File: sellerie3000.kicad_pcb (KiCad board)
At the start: 2 copper layers, 25.4 x 10.2 mm, 19 parts, among them J1 USB_C_Receptacle, J2 Conn_01x04, J3 Conn_01x02, J4 Conn_01x02, U1 FT230XQ-R

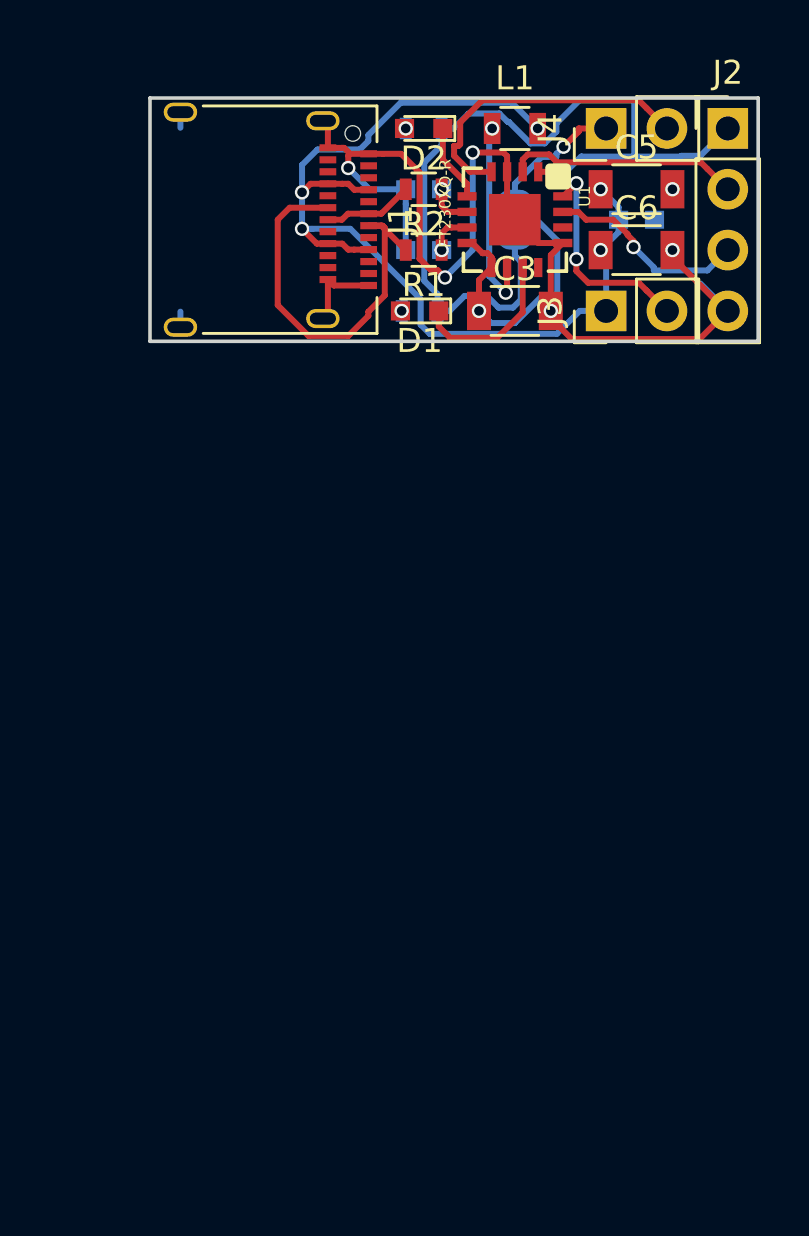
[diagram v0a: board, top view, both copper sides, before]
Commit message: wow much update many unfinished
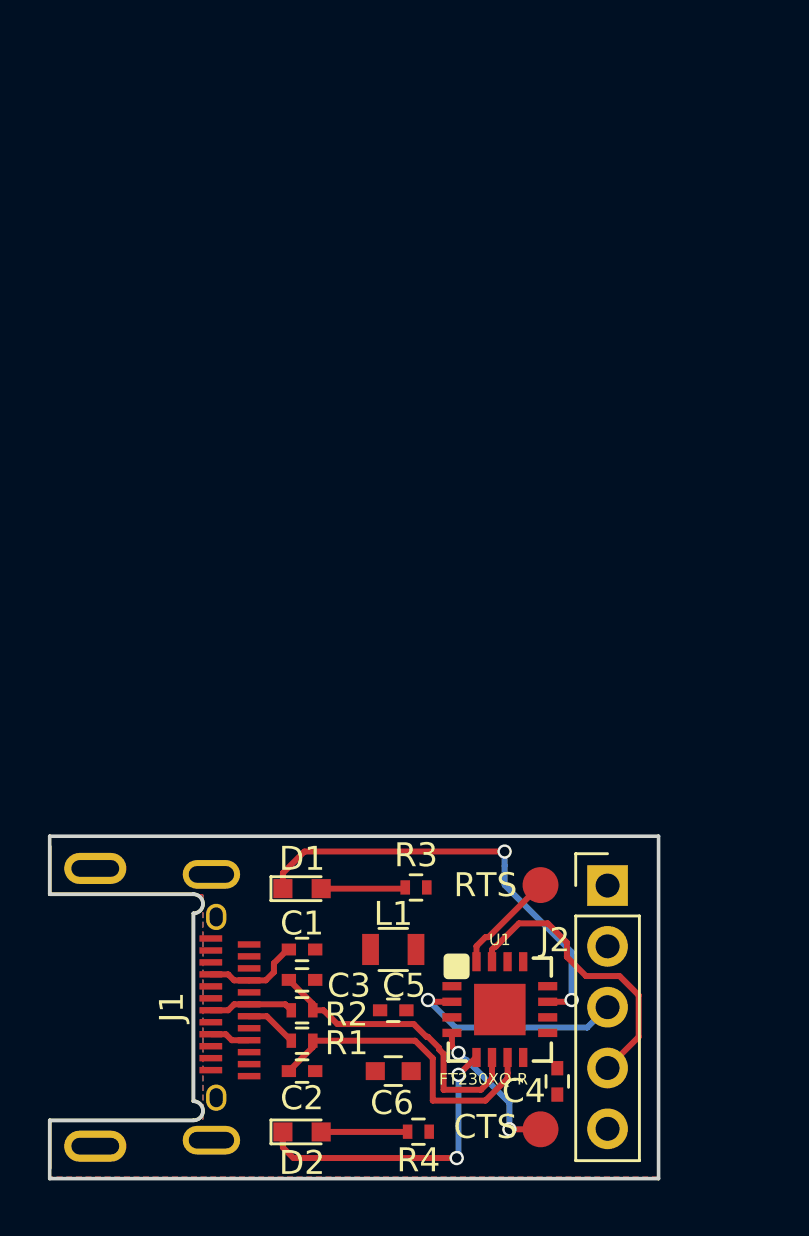
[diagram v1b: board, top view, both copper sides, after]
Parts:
- removed J3, J4: Conn_01x02, Pin_Headers:Pin_Header_Straight_1x02_Pitch2.54mm
- removed JP1: VMODE, sellerie3000:Solder_Jumper
- added CTS: CTS, Measurement_Points:Measurement_Point_Round-SMD-Pad_Small, F.Cu at (139.5, 143.4)
- added RTS: RTS, Measurement_Points:Measurement_Point_Round-SMD-Pad_Small, F.Cu at (139.5, 133.2)
- C1: value 47pF -> 10nF; footprint Capacitors_SMD:C_0603 -> Capacitors_SMD:C_0402; moved to F.Cu
- C2: footprint Capacitors_SMD:C_0603 -> Capacitors_SMD:C_0402; moved to F.Cu
- C3: value 100nF -> 47pF; footprint Capacitors_SMD:C_1206 -> Capacitors_SMD:C_0402
- C4: value 10nF -> 100nF; footprint Capacitors_SMD:C_0603 -> Capacitors_SMD:C_0402; moved to F.Cu
- C5: footprint Capacitors_SMD:C_1206 -> Capacitors_SMD:C_0402
- C6: footprint Capacitors_SMD:C_1206 -> Capacitors_SMD:C_0603
- D1: value RXLED -> RX
- D2: value TXLED -> TX
- J1: footprint Connectors_USB:USB_C_Receptacle_Amphenol_12401610E4-2A -> DX07B024JJ3:DX07B024JJ3
- J2: value Conn_01x04 -> Conn_01x05; footprint Pin_Headers:Pin_Header_Straight_1x04_Pitch2.54mm -> Pin_Headers:Pin_Header_Straight_1x05_Pitch2.54mm
- R1, R2: footprint Resistors_SMD:R_0603 -> Resistors_SMD:R_0402
- R3, R4: footprint Resistors_SMD:R_0603 -> Resistors_SMD:R_0402; moved to F.Cu
- moved D2 42.2 mm to (129.5, 143.5), turned to 0 degrees
- moved R4 41.9 mm to (134.4, 143.5)
- moved C4 36.1 mm to (140.2, 141.4), turned to 270 degrees
- moved C5 35.8 mm to (133.3, 138.4)
- moved C6 35.8 mm to (133.3, 141.0)
- moved R2 34.7 mm to (129.5, 138.4)
- moved C2 34.7 mm to (129.5, 141.0), turned to 0 degrees
- moved L1 34.7 mm to (133.3, 135.9)
- moved R1 33.4 mm to (129.5, 139.7)
- moved U1 33.0 mm to (137.8, 138.4), turned to 0 degrees
- moved J1 32.9 mm to (125.8, 138.3)
- moved C1 32.2 mm to (129.5, 135.9), turned to 0 degrees
- moved J2 32.0 mm to (142.3, 133.2)
- moved C3 29.3 mm to (129.5, 137.2)
- moved D1 24.6 mm to (129.5, 133.3), turned to 0 degrees
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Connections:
- net CBUS1 renamed /CBUS1
- net CBUS2 renamed /CBUS2
- net Net-(C2-Pad1) renamed /USBDM
- C3 pad 1: 3V3 -> /USBDP
- C4 pad 1: VCC -> 3V3
- J1 pad A4: VCC -> Net-(C1-Pad1)
- J1 pad A9: VCC -> Net-(C1-Pad1)
- J1 pad B4: VCC -> Net-(C1-Pad1)
- J1 pad B9: VCC -> Net-(C1-Pad1)
- J2 pad 1: VCCIO -> VCC
- J2 pad 2: RX -> 3V3
- J2 pad 3: TX -> RX
- J2 pad 4: GND -> TX
- L1 pad 1: Net-(L1-Pad1) -> VCC
- L1 pad 2: VCC -> Net-(C1-Pad1)
- R2 pad 1: Net-(C1-Pad1) -> /USBDP
- R3 pad 1: VCCIO -> 3V3
- R4 pad 1: VCCIO -> 3V3
- U1 pad 1: VCCIO -> 3V3
- U1 pad 10: Net-(L1-Pad1) -> VCC
- U1 pad 16: RTS -> /RTS
- U1 pad 4: CTS -> /CTS
- U1 pad 6: Net-(C1-Pad1) -> /USBDP
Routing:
- net GND: track 50.3 -> 0.00 mm, vias 6 -> 0
- net VCC: track 41.7 -> 0.00 mm, vias 5 -> 0
- net VCCIO: track 36.0 -> 0.00 mm, vias 1 -> 0
- net 3V3: track 18.2 -> 0.00 mm, vias 2 -> 0
- net Net-(J1-PadA7): track 17.2 -> 2.18 mm
- net CTS: track 13.0 -> 0.00 mm
- net /USBDP: track 0.00 -> 12.5 mm
- net /CBUS1: track 6.66 -> 18.7 mm, vias 0 -> 2
- net /USBDM: track 1.86 -> 13.1 mm, vias 1 -> 0
- net /CBUS2: track 3.25 -> 12.6 mm, vias 0 -> 2
- net RTS: track 8.93 -> 0.00 mm, vias 2 -> 0
- net Net-(L1-Pad1): track 8.27 -> 0.00 mm, vias 2 -> 0
- net /CTS: track 0.00 -> 6.35 mm, vias 0 -> 2
- net /RTS: track 0.00 -> 4.38 mm
- net Net-(C1-Pad1): track 1.86 -> 5.82 mm, vias 1 -> 0
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- added copper zone on F.Cu, net GND
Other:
- board size 25.4 x 10.2 mm -> 25.4 x 14.3 mm

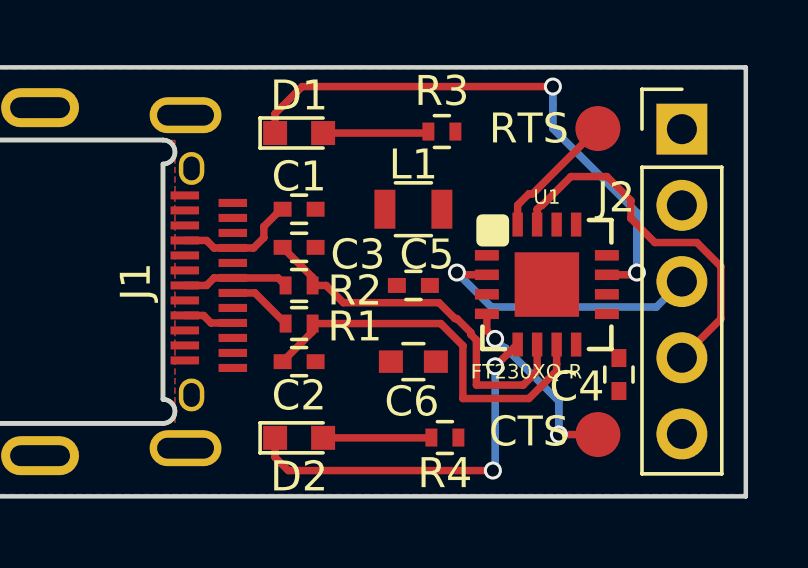
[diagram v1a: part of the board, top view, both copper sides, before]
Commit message: nearly done
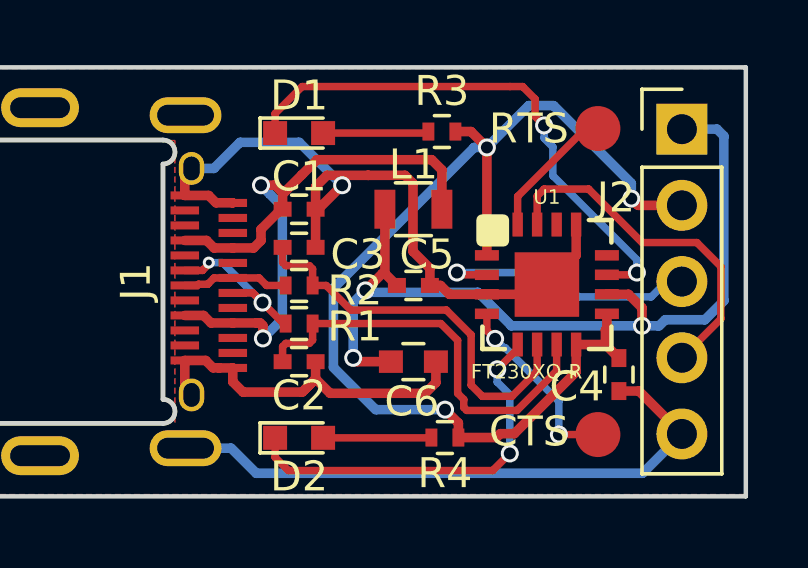
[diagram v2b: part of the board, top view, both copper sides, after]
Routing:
- net GND: track 0.00 -> 58.4 mm, vias 0 -> 1
- net 3V3: track 0.00 -> 37.1 mm, vias 0 -> 3
- net VCC: track 0.00 -> 29.0 mm, vias 0 -> 3
- net Net-(C1-Pad1): track 5.82 -> 23.5 mm, vias 0 -> 2
- net Net-(J1-PadA7): track 2.18 -> 5.47 mm, vias 0 -> 2
- net /USBDM: track 13.1 -> 14.1 mm
- net /USBDP: track 12.5 -> 13.4 mm
- net /CBUS1: track 18.7 -> 18.1 mm
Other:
- net class Power added: clearance 0.2, trace_width 0.32, via_dia 0.6, via_drill 0.4
